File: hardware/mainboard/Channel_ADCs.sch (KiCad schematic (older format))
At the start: 58 parts, among them J10 VOL_B, J11 PITCH_C, J12 PITCH_D, J13 VOL_C, J14 VOL_D, J7 PITCH_A, J8 PITCH_B, J9 VOL_A, U8 MAX11300_TQFP, U9 MAX11300_TQFP

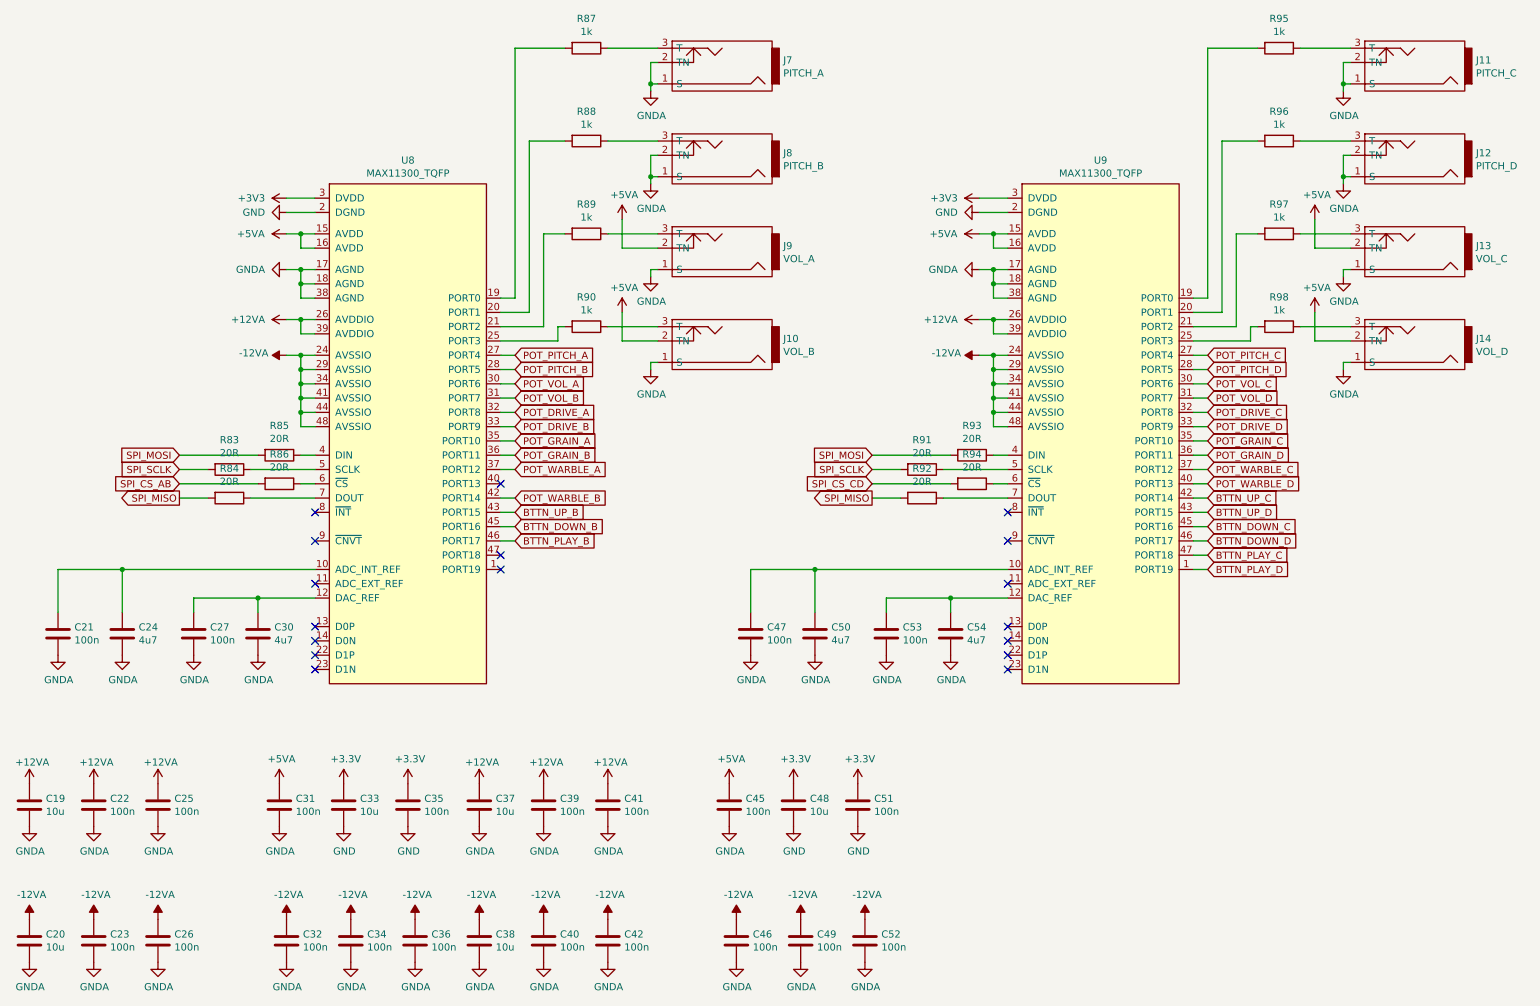
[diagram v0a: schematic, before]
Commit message: hardware: update schematics & add BOM
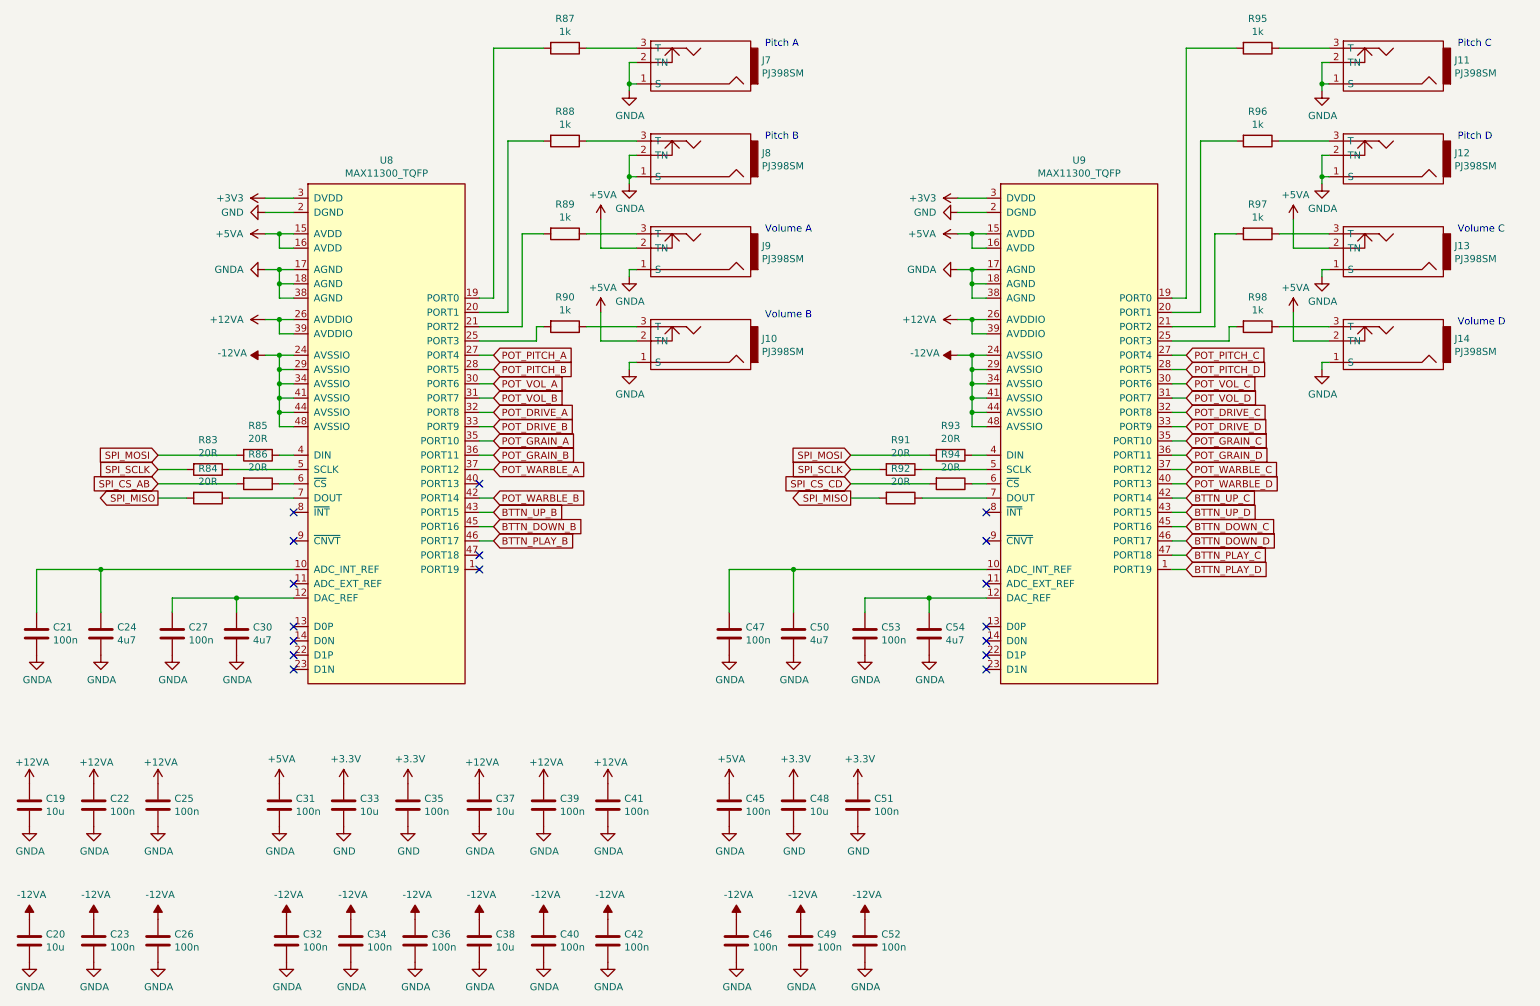
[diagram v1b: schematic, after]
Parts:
- J10: value VOL_B -> PJ398SM
- J11: value PITCH_C -> PJ398SM
- J12: value PITCH_D -> PJ398SM
- J13: value VOL_C -> PJ398SM
- J14: value VOL_D -> PJ398SM
- J7: value PITCH_A -> PJ398SM
- J8: value PITCH_B -> PJ398SM
- J9: value VOL_A -> PJ398SM
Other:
- note added: "Pitch A"
- note added: "Pitch B"
- note added: "Pitch C"
- note added: "Pitch D"
- note added: "Volume A"
- note added: "Volume B"
- note added: "Volume C"
- note added: "Volume D"
- moved on the sheet: C21, C24, C27, C30, C47, C50, C53, C54, J10, J11, J12, J13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
